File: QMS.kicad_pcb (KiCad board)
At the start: 2 copper layers, 48.1 x 33 mm, 4 parts, among them J1 Screw_Terminal_01x02, U1 ESP-12E, U2 AMS1117-3.3

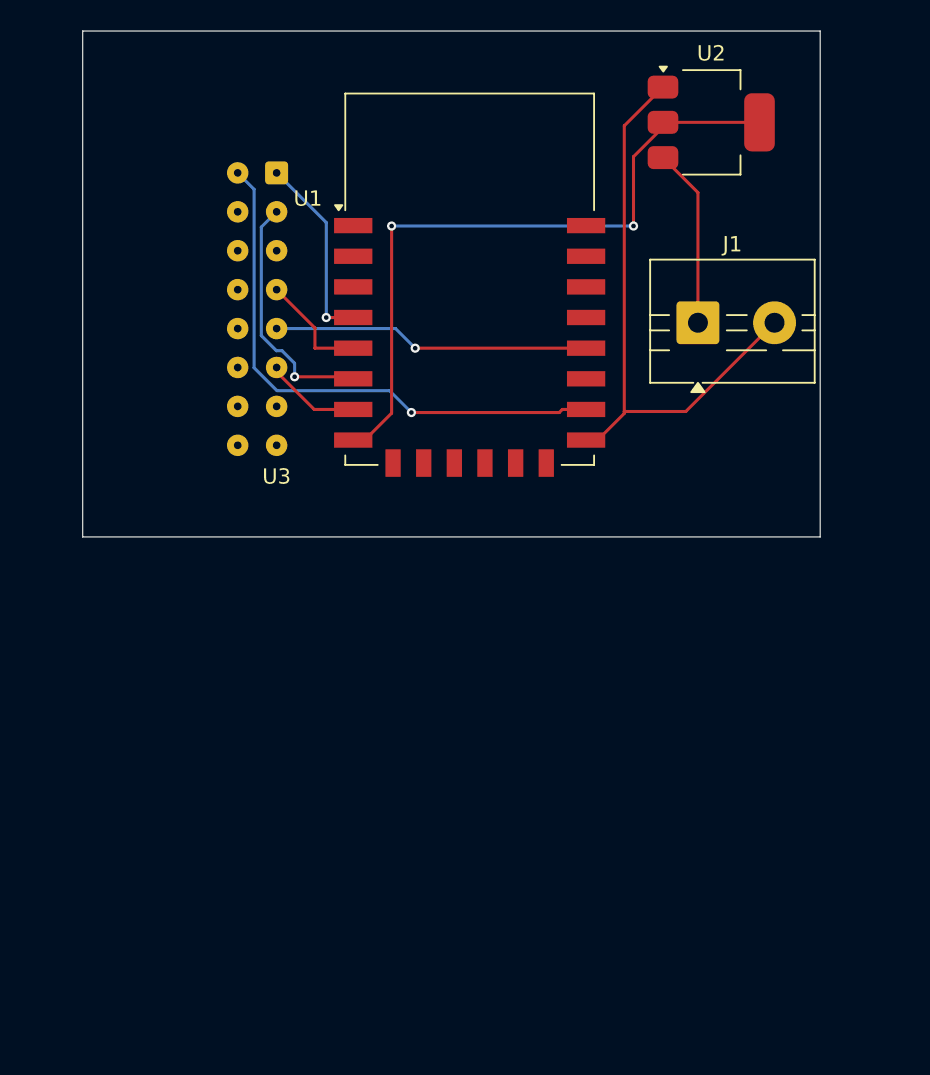
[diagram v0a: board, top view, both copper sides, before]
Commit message: least
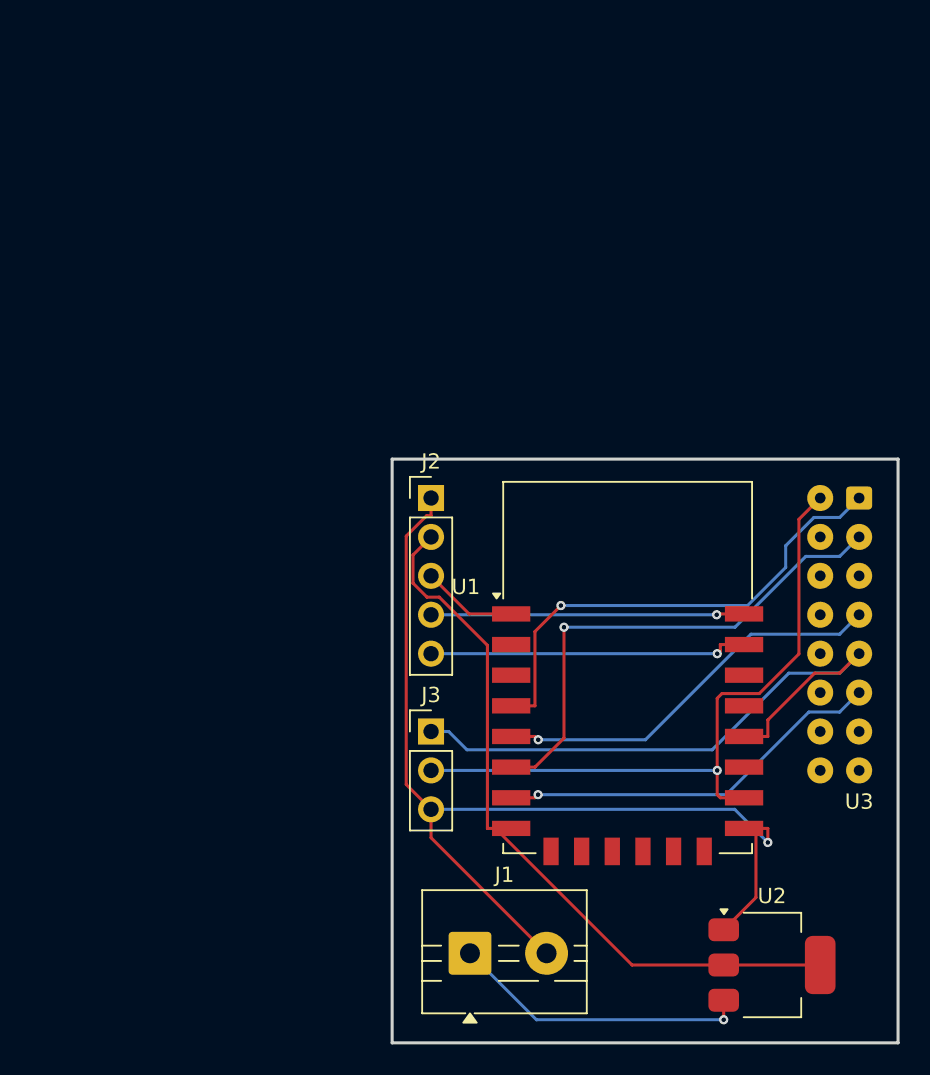
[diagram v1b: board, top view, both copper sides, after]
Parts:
- added J2: PINHD_1x5_Male, Connector_PinHeader_2.54mm:PinHeader_1x05_P2.54mm_Vertical, F.Cu at (132.1, 91.4)
- added J3: PINHD_1x3_Male, Connector_PinHeader_2.54mm:PinHeader_1x03_P2.54mm_Vertical, F.Cu at (132.1, 106.7)
- moved U2 55.1 mm to (154.3, 121.9)
- moved J1 43.8 mm to (134.6, 121.2)
- moved U3 43.5 mm to (160.0, 111.8)
- moved U1 27.4 mm to (144.9, 102.5)
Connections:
- U1 pad 1: unconnected-(U1-~{RST}-Pad1) -> Net-(U1-~{RST})
- U1 pad 21: unconnected-(U1-GPIO3/RXD-Pad21) -> Net-(U1-GPIO3/RXD)
- U1 pad 22: unconnected-(U1-GPIO1/TXD-Pad22) -> Net-(U1-GPIO1/TXD)
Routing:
- net GND: track 37.8 -> 67.2 mm, vias 0 -> 1
- net Net-(U1-GPIO3/RXD): track 0.00 -> 20.9 mm, vias 0 -> 1
- net Net-(U1-GPIO0): track 20.7 -> 41.4 mm, vias 1 -> 0
- net Net-(U1-GPIO1/TXD): track 0.00 -> 20.5 mm, vias 0 -> 1
- net Net-(U1-GPIO16): track 12.5 -> 32.0 mm
- net Net-(U1-GPIO13): track 6.30 -> 25.6 mm, vias 0 -> 1
- net Net-(U1-GPIO14): track 7.36 -> 26.2 mm, vias 0 -> 1
- net Net-(U1-GPIO12): track 16.2 -> 33.2 mm
- net Net-(U1-GPIO15): track 36.1 -> 44.1 mm
- net Net-(J1-Pin_1): track 11.7 -> 19.6 mm, vias 0 -> 1
- net Net-(U1-~{RST}): track 0.00 -> 6.26 mm
- net Net-(U1-VCC): track 45.2 -> 48.4 mm, vias 2 -> 0
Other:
- board size 48.1 x 33 mm -> 33 x 38.1 mm

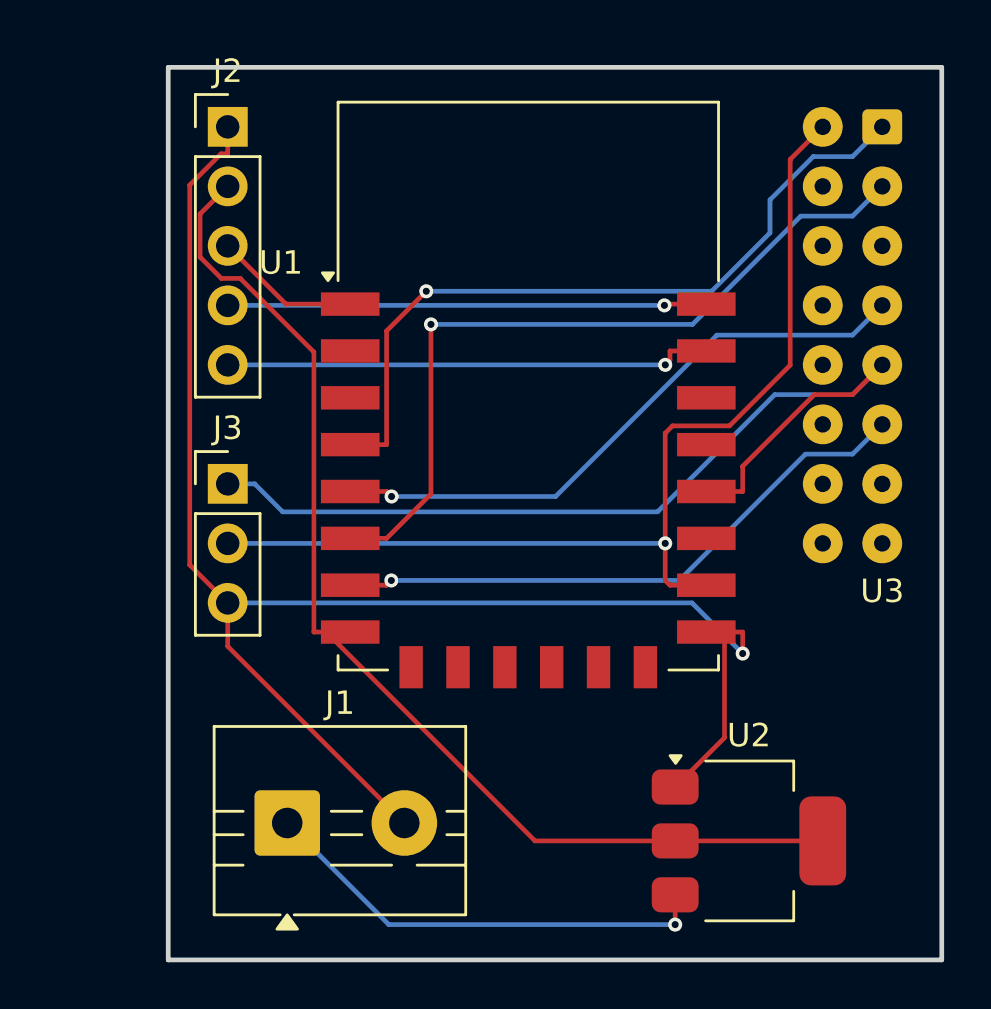
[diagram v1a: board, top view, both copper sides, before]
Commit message: complete
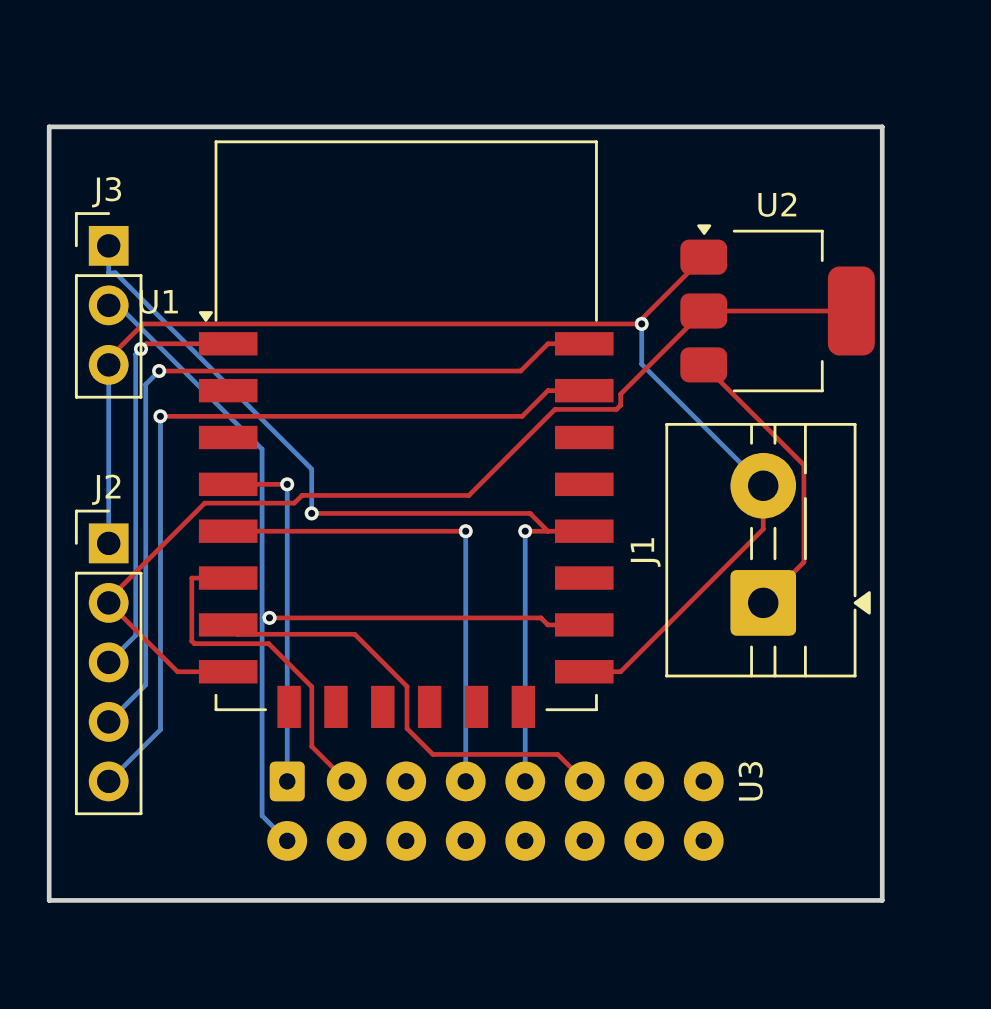
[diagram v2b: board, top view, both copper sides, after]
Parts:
- moved U2 22.7 mm to (155.6, 99.3)
- moved J1 22.4 mm to (154.9, 111.8), turned to 90 degrees
- moved J2 18.5 mm to (127.0, 109.2)
- moved J3 11.4 mm to (127.0, 96.5)
- moved U3 9.16 mm to (154.9, 119.4), turned to 90 degrees
- moved U1 5.48 mm to (139.7, 104.2)
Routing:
- net Net-(U1-GPIO12): track 33.2 -> 14.8 mm, vias 1 -> 0
- net Net-(U1-GPIO16): track 32.0 -> 15.2 mm
- net Net-(U1-GPIO3/RXD): track 20.9 -> 35.0 mm
- net Net-(U1-GPIO1/TXD): track 20.5 -> 34.5 mm
- net Net-(U1-~{RST}): track 6.26 -> 17.8 mm, vias 0 -> 1
- net GND: track 67.2 -> 56.3 mm
- net Net-(J1-Pin_1): track 19.6 -> 12.7 mm, vias 1 -> 0
- net Net-(U1-GPIO13): track 25.6 -> 19.0 mm, vias 1 -> 0
- net Net-(U1-GPIO14): track 26.2 -> 20.8 mm
- net Net-(U1-VCC): track 48.4 -> 43.6 mm
- net Net-(U1-GPIO15): track 44.1 -> 40.1 mm
- net Net-(U1-GPIO0): track 41.4 -> 38.8 mm, vias 0 -> 2
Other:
- board size 33 x 38.1 mm -> 35.6 x 33 mm

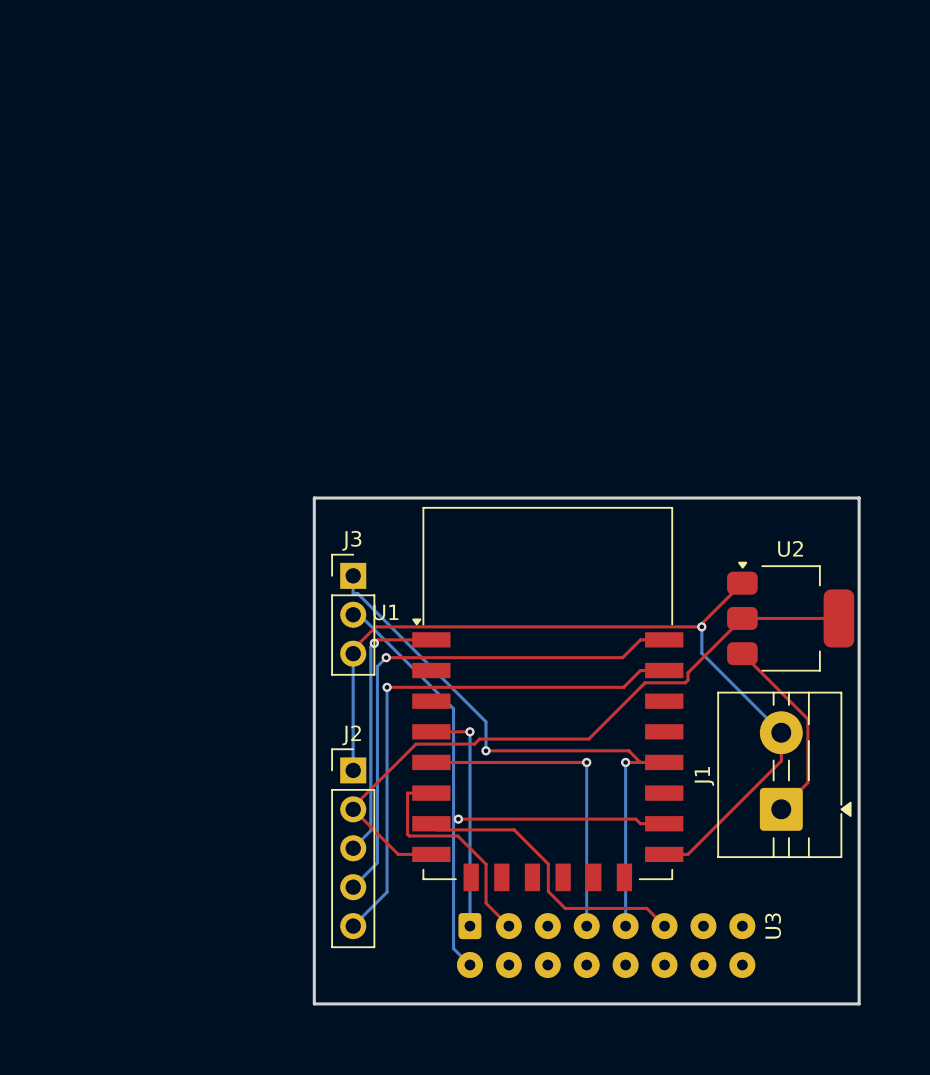
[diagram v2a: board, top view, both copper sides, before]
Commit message: completed
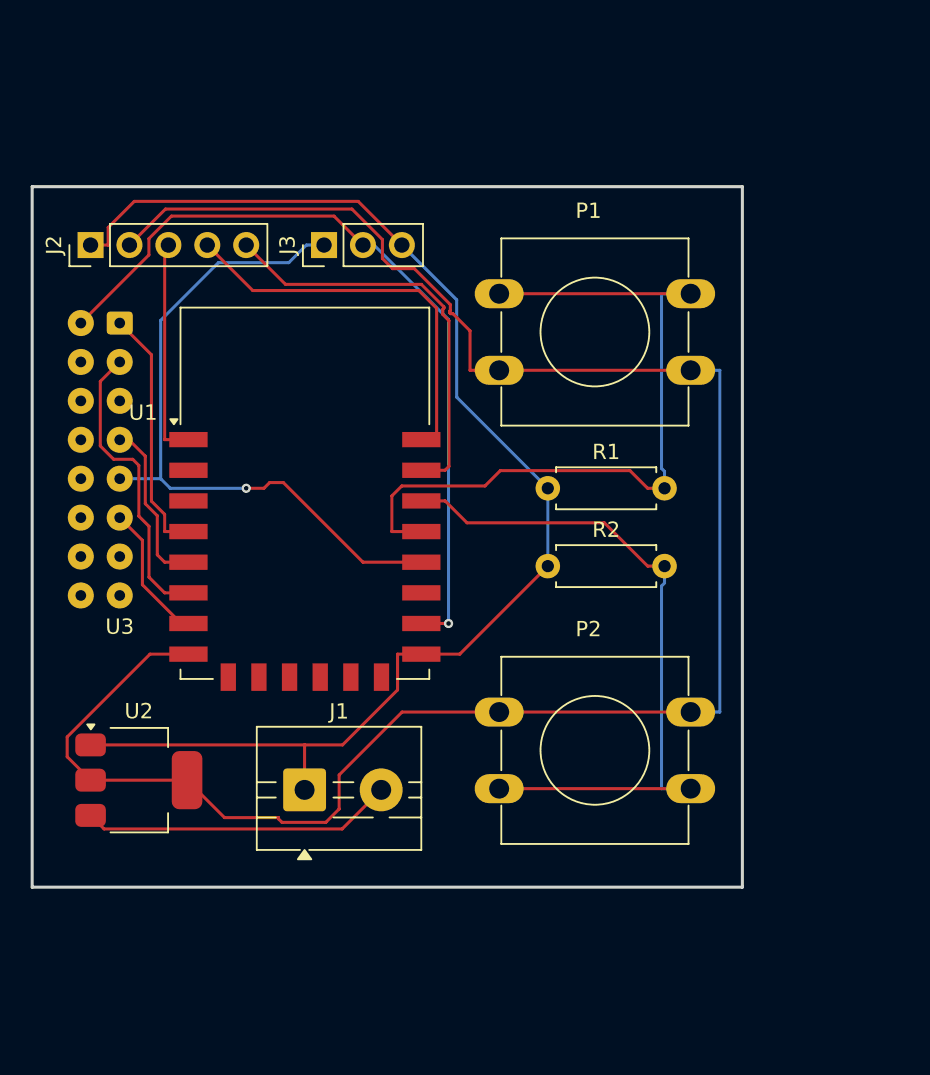
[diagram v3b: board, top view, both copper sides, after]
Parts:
- added P1: ~, Button_Switch_THT:SW_PUSH-12mm, F.Cu at (136.5, 78.1)
- added P2: ~, Button_Switch_THT:SW_PUSH-12mm, F.Cu at (136.5, 105.4)
- added R1: Resistor, Resistor_THT:R_Axial_DIN0207_L6.3mm_D2.5mm_P7.62mm_Horizontal, F.Cu at (139.7, 90.8)
- added R2: Resistor, Resistor_THT:R_Axial_DIN0207_L6.3mm_D2.5mm_P7.62mm_Horizontal, F.Cu at (139.7, 95.9)
- moved U3 47.2 mm to (111.8, 100.3), turned to 0 degrees
- moved U2 43.8 mm to (113.0, 109.9)
- moved J2 38.3 mm to (109.9, 74.9), turned to 90 degrees
- moved J1 31.1 mm to (123.8, 110.5), turned to 0 degrees
- moved J3 21.7 mm to (125.1, 74.9), turned to 90 degrees
- moved U1 20.5 mm to (123.8, 91.1)
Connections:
- net Net-(U1-GPIO1/TXD) renamed /TX
- net Net-(U1-GPIO3/RXD) renamed /RX
- net Net-(U1-VCC) renamed /VCC 3.3v
- net Net-(U1-~{RST}) renamed /RESET
- J1 pad 1: Net-(J1-Pin_1) -> GND
- J1 pad 2: GND -> Net-(J1-Pin_2)
- U1 pad 19: unconnected-(U1-GPIO4-Pad19) -> Net-(U1-GPIO4)
- U1 pad 20: unconnected-(U1-GPIO5-Pad20) -> Net-(U1-GPIO5)
- U2 pad 3: Net-(J1-Pin_1) -> Net-(J1-Pin_2)
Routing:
- net /VCC 3.3v: track 43.6 -> 128.9 mm
- net Net-(U1-GPIO4): track 0.00 -> 50.4 mm
- net Net-(U1-GPIO5): track 0.00 -> 46.6 mm
- net GND: track 56.3 -> 87.2 mm, vias 1 -> 0
- net Net-(J1-Pin_2): track 0.00 -> 20.4 mm
- net Net-(J1-Pin_1): track 12.7 -> 0.00 mm
- net Net-(U1-GPIO15): track 40.1 -> 51.9 mm
- net Net-(U1-GPIO13): track 19.0 -> 9.05 mm
- net Net-(U1-GPIO14): track 20.8 -> 11.1 mm, vias 1 -> 0
- net /TX: track 34.5 -> 26.2 mm, vias 1 -> 0
- net /RX: track 35.0 -> 27.1 mm, vias 1 -> 0
- net Net-(U1-GPIO0): track 38.8 -> 45.3 mm, vias 2 -> 1
- net Net-(U1-GPIO12): track 14.8 -> 19.6 mm
- net /RESET: track 17.8 -> 14.4 mm, vias 1 -> 0
- net Net-(U1-GPIO16): track 15.2 -> 16.4 mm, vias 1 -> 0
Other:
- board size 35.6 x 33 mm -> 46.4 x 45.7 mm
